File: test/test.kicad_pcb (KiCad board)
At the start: 2 copper layers, 8.9 x 7.6 mm, 2 parts, among them J1 Conn_01x03_Male, Q1 Q_NJFET_DGS

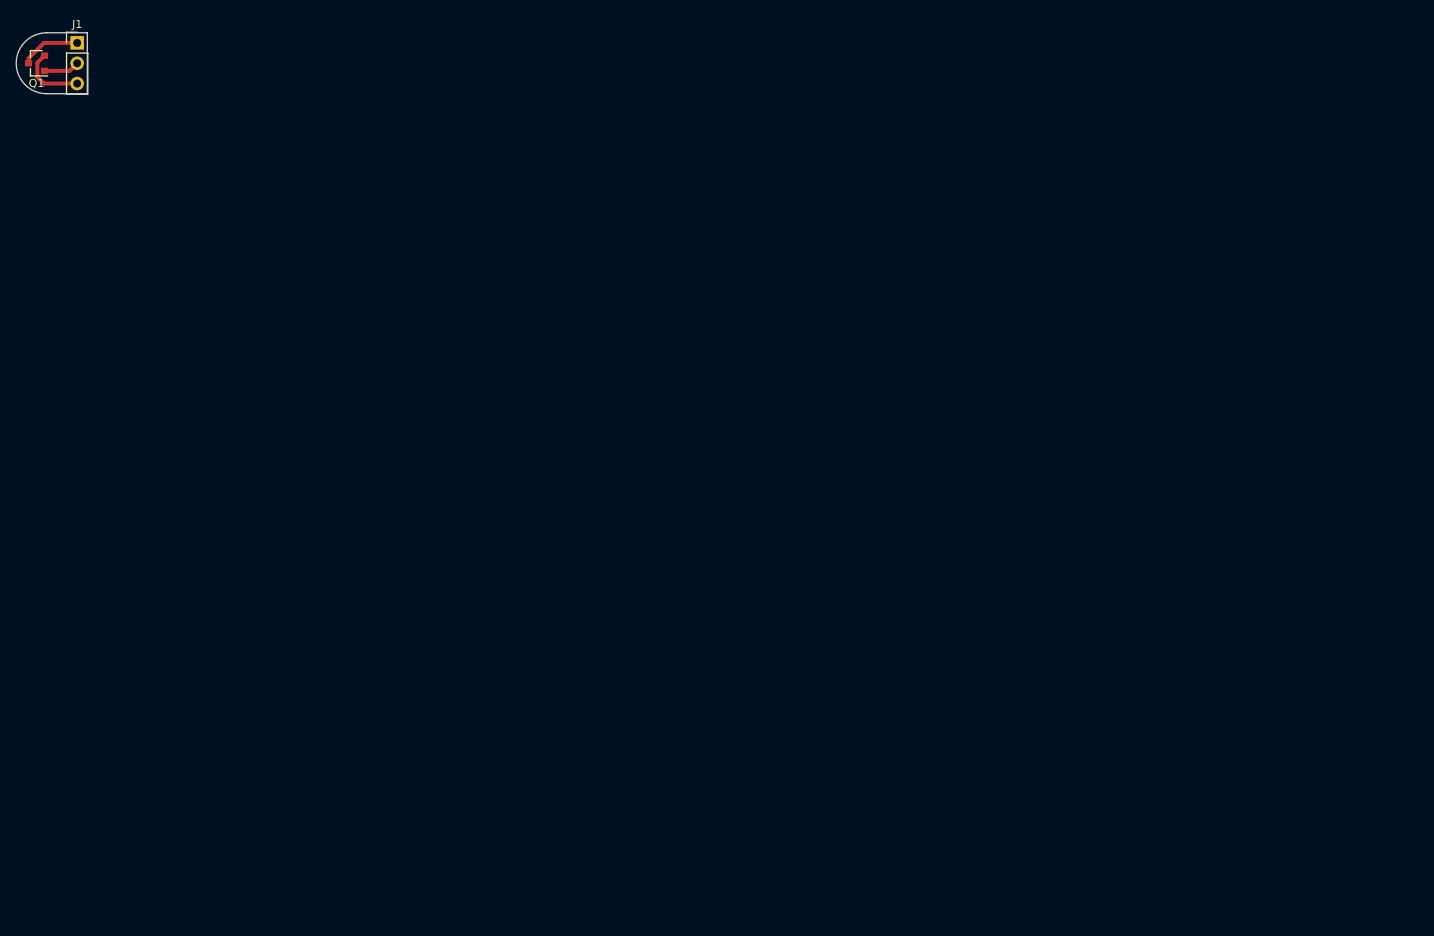
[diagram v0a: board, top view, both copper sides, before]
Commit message: work on test and clip mix
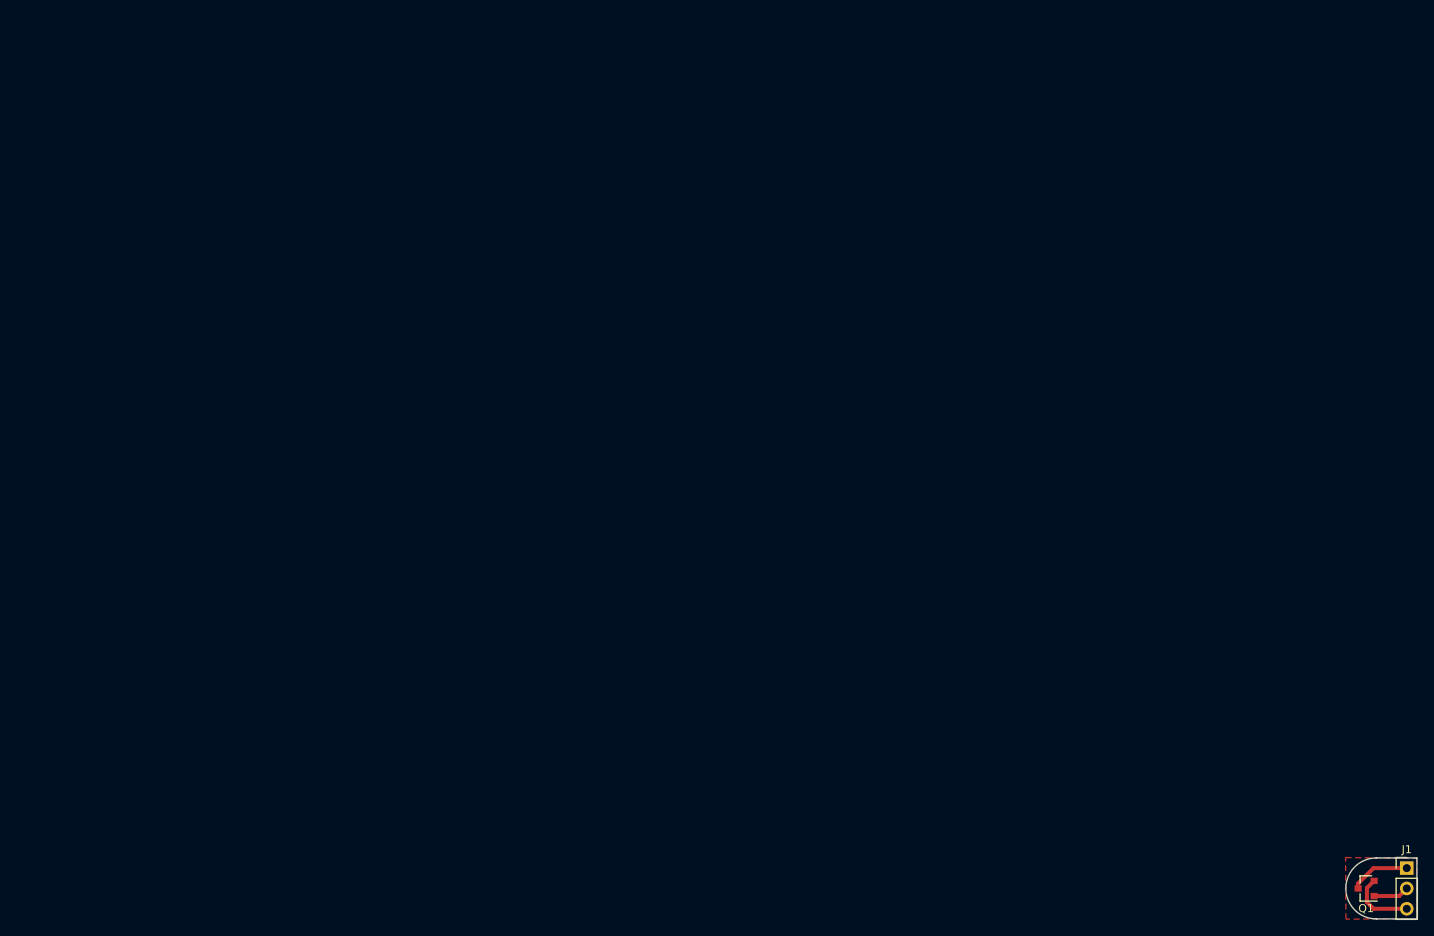
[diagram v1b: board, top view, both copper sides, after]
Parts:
- moved Q1 195.6 mm to (170.4, 108.6)
- moved J1 195.6 mm to (175.4, 106.1)
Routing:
- added copper zone on F.Cu, net (none)
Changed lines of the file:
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@@
   (general
     (thickness 1.6)
-    (drawings 5)
+    (drawings 4)
     (tracks 9)
     (zones 0)
@@
     (pad_drill 0.762)
     (pad_to_mask_clearance 0)
-    (aux_axis_origin 0 0)
+    (aux_axis_origin 167.8 104.75)
     (visible_elements 7FFFFFFF)
     (pcbplotparams
-      (layerselection 0x00000_7fffffff)
+      (layerselection 0x01000_7fffffff)
       (usegerberextensions false)
       (usegerberattributes true)
@@
   )
   (module Package_TO_SOT_SMD:SOT-23 (layer F.Cu)
-    (at 4.17 5.46 180)
+    (at 170.37 108.61 180)
     (descr "SOT-23, Standard")
     (tags SOT-23)
@@
   )
   (module Connector_PinHeader_2.54mm:PinHeader_1x03_P2.54mm_Vertical (layer F.Cu)
-    (at 9.25 2.92)
+    (at 175.45 106.07)
     (descr "Through hole straight pin header, 1x03, 2.54mm pitch, single row")
     (tags "Through hole pin header THT 1x03 2.54mm single row")
@@
     )
   )
-  (target plus (at 1.63 1.65) (size 5) (width 0.05) (layer Edge.Cuts))
-  (gr_line (start 10.52 1.65) (end 10.52 9.27) (layer Edge.Cuts) (width 0.05))
-  (gr_arc (start 5.44 5.46) (end 5.44 1.65) (angle -180) (layer Edge.Cuts) (width 0.05))
-  (gr_line (start 10.52 1.65) (end 5.44 1.65) (layer Edge.Cuts) (width 0.05))
-  (gr_line (start 10.52 9.27) (end 5.44 9.27) (layer Edge.Cuts) (width 0.05))
-  (segment (start 5.099998 8) (end 9.25 8) (width 0.5) (layer F.Cu) (net 1))
-  (segment (start 4.269999 7.170001) (end 5.099998 8) (width 0.5) (layer F.Cu) (net 1))
-  (segment (start 4.269999 5.410001) (end 4.269999 7.170001) (width 0.5) (layer F.Cu) (net 1))
-  (segment (start 5.17 4.51) (end 4.269999 5.410001) (width 0.5) (layer F.Cu) (net 1))
-  (segment (start 8.3 6.41) (end 9.25 5.46) (width 0.5) (layer F.Cu) (net 2))
-  (segment (start 5.17 6.41) (end 8.3 6.41) (width 0.5) (layer F.Cu) (net 2))
-  (segment (start 3.17 4.849998) (end 3.17 5.46) (width 0.5) (layer F.Cu) (net 3))
-  (segment (start 5.099998 2.92) (end 3.17 4.849998) (width 0.5) (layer F.Cu) (net 3))
-  (segment (start 9.25 2.92) (end 5.099998 2.92) (width 0.5) (layer F.Cu) (net 3))
+  (gr_line (start 176.72 104.8) (end 176.72 112.42) (layer Edge.Cuts) (width 0.05))
+  (gr_arc (start 171.64 108.61) (end 171.64 104.8) (angle -180) (layer Edge.Cuts) (width 0.05))
+  (gr_line (start 176.72 104.8) (end 171.64 104.8) (layer Edge.Cuts) (width 0.05))
+  (gr_line (start 176.72 112.42) (end 171.64 112.42) (layer Edge.Cuts) (width 0.05))
+  (segment (start 171.299998 111.15) (end 175.45 111.15) (width 0.5) (layer F.Cu) (net 1))
+  (segment (start 170.469999 110.320001) (end 171.299998 111.15) (width 0.5) (layer F.Cu) (net 1))
+  (segment (start 170.469999 108.560001) (end 170.469999 110.320001) (width 0.5) (layer F.Cu) (net 1))
+  (segment (start 171.37 107.66) (end 170.469999 108.560001) (width 0.5) (layer F.Cu) (net 1))
+  (segment (start 174.5 109.56) (end 175.45 108.61) (width 0.5) (layer F.Cu) (net 2))
+  (segment (start 171.37 109.56) (end 174.5 109.56) (width 0.5) (layer F.Cu) (net 2))
+  (segment (start 169.37 107.999998) (end 169.37 108.61) (width 0.5) (layer F.Cu) (net 3))
+  (segment (start 171.299998 106.07) (end 169.37 107.999998) (width 0.5) (layer F.Cu) (net 3))
+  (segment (start 175.45 106.07) (end 171.299998 106.07) (width 0.5) (layer F.Cu) (net 3))
+  (zone (net 0) (net_name "") (layer F.Cu) (hatch edge 0.508)
+    (connect_pads (clearance 0.508))
+    (min_thickness 0.254)
+    (fill yes (arc_segments 32) (thermal_gap 0.508) (thermal_bridge_width 0.508))
+    (polygon
+      (pts
+        (xy 176.7 104.85) (xy 176.75 112.4) (xy 167.85 112.45) (xy 167.8 104.75)
+      )
+    )
+  )
 )
